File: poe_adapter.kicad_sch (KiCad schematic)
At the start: 27 parts, among them J1 USB_C_Receptacle, J2 RJ45_LED_Shielded, U1 LM2575HVS

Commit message: Update PCB
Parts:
- J1: footprint (none) -> Connector_USB:USB_C_Receptacle_Amphenol_12401610E4-2A_CircularHoles
- U1: footprint KTT0005B -> PoE_Devices:LM2575HVS-12

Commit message: PCB Design Rule updated
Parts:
- C11: footprint Capacitor_SMD:CP_Elec_18x17.5 -> Capacitor_SMD:CP_Elec_8x10
- J2: footprint Connector_RJ:RJ45_Amphenol_RJHSE5380 -> Connector_RJ:RJ45_Amphenol_RJHSE538X
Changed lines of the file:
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@@
       (effects (font (size 1.27 1.27)) (justify left))
     )
-    (property "Footprint" "Capacitor_SMD:CP_Elec_18x17.5" (id 2) (at 150.495 146.685 0)
+    (property "Footprint" "Capacitor_SMD:CP_Elec_8x10" (id 2) (at 150.495 146.685 0)
       (effects (font (size 1.27 1.27)) hide)
     )
@@
     (property "Reference" "J2" (id 0) (at 50.165 21.59 0))
     (property "Value" "RJ45_LED_Shielded" (id 1) (at 50.165 24.13 0))
-    (property "Footprint" "Connector_RJ:RJ45_Amphenol_RJHSE5380" (id 2) (at 50.165 38.735 90)
+    (property "Footprint" "Connector_RJ:RJ45_Amphenol_RJHSE538X" (id 2) (at 50.165 38.735 90)
       (effects (font (size 1.27 1.27)) hide)
     )
@@
     )
     (path "/175d2401-eed6-416a-938c-46d3b5f22d0e"
-      (reference "C11") (unit 1) (value "330uF") (footprint "Capacitor_SMD:CP_Elec_18x17.5")
+      (reference "C11") (unit 1) (value "330uF") (footprint "Capacitor_SMD:CP_Elec_8x10")
     )
     (path "/9d43f031-4287-4645-997e-8ec53611a4dd/8805b2c8-4492-42ee-9738-f7deb31ea902"
@@
     )
     (path "/30ad6084-9389-411c-add3-d2b2fd2e6d22"
-      (reference "J2") (unit 1) (value "RJ45_LED_Shielded") (footprint "Connector_RJ:RJ45_Amphenol_RJHSE5380")
+      (reference "J2") (unit 1) (value "RJ45_LED_Shielded") (footprint "Connector_RJ:RJ45_Amphenol_RJHSE538X")
     )
     (path "/51efc304-0253-4cf9-b8a4-37a603089f63/20b2cc4c-dd50-47a4-a2f0-3800c15edb7c"

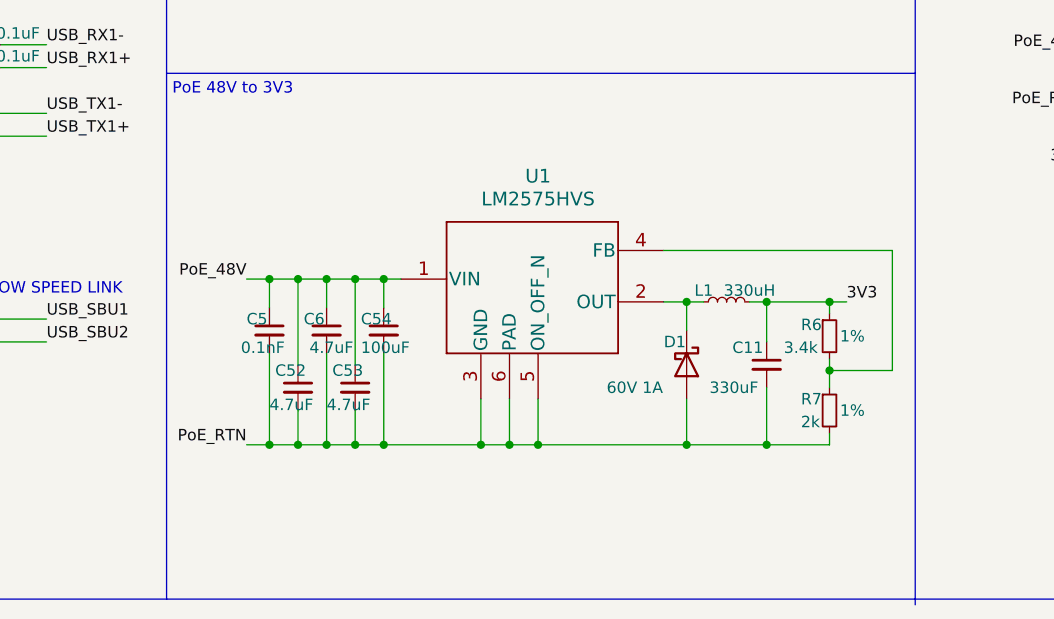
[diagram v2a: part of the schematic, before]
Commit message: Update 3V3 Solution
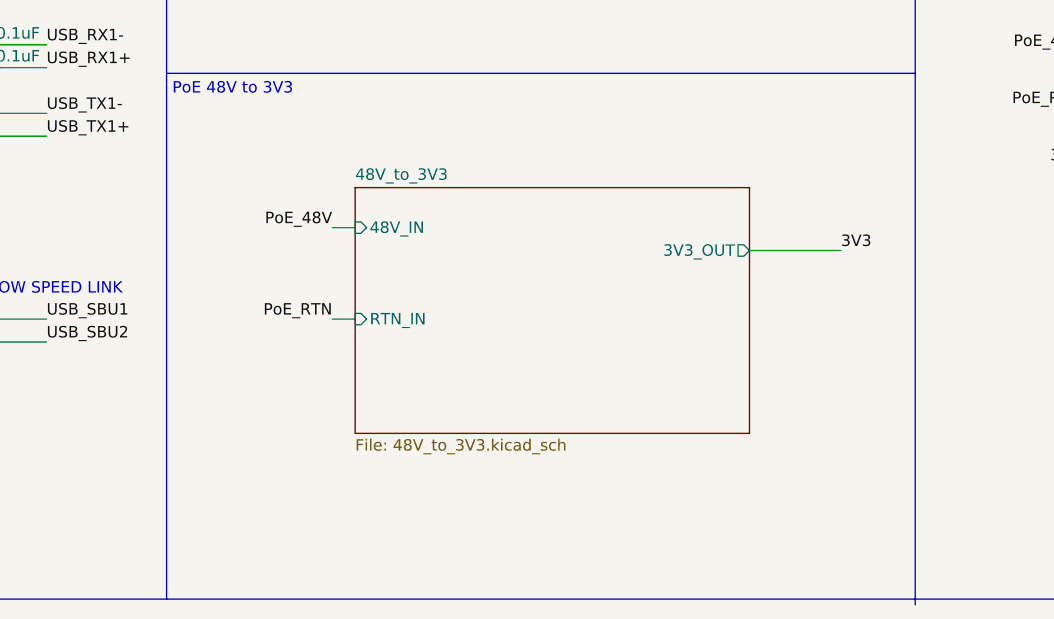
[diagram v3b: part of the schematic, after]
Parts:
- removed C11: 330uF, Capacitor_SMD:CP_Elec_8x10, symbol Device:C_Small
- removed C5: 0.1nF, Capacitor_SMD:C_0603_1608Metric, symbol Device:C_Small
- removed C52, C53, C6: 4.7uF, Capacitor_SMD:C_1206_3216Metric, symbol Device:C_Small
- removed C54: 100uF, Capacitor_SMD:CP_Elec_10x10, symbol Device:C_Small
- removed D1: 60V 1A, Diode_SMD:D_SMA, symbol Device:D_Schottky
- removed L1: 330uH, Inductor_SMD:L_12x12mm_H8mm, symbol Device:L_Small
- removed R6: 3.4k, Resistor_SMD:R_0603_1608Metric, symbol Device:R_Small
- removed R7: 2k, Resistor_SMD:R_0603_1608Metric, symbol Device:R_Small
- removed U1: LM2575HVS, PoE_Devices:LM2575HVS-12, symbol LM2575HV:LM2575HVS
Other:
- added sheet 48V_to_3V3 (48V_to_3V3.kicad_sch)
